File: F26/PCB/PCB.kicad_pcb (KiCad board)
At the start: 2 copper layers, 12 parts, among them J1 B3B-XH-A, J3 B2B-XH-A, J4 B3B-XH-A, J5 Conn_01x04, J6 Conn_01x06, J7 Conn_01x02, SW1 SW_Nidec_CAS-120A1, U4 815, U6 SC0194_9_

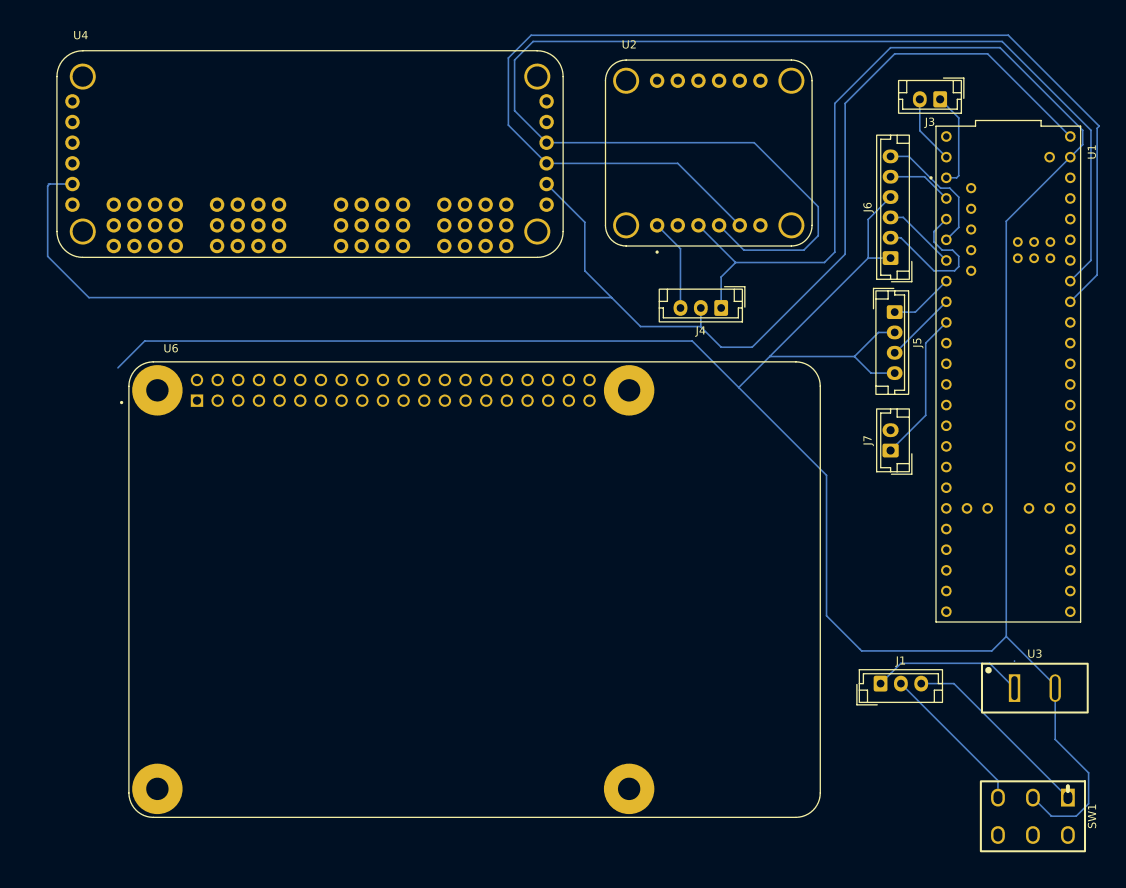
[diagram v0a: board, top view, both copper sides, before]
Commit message: PCB updates and Made wiring diagram
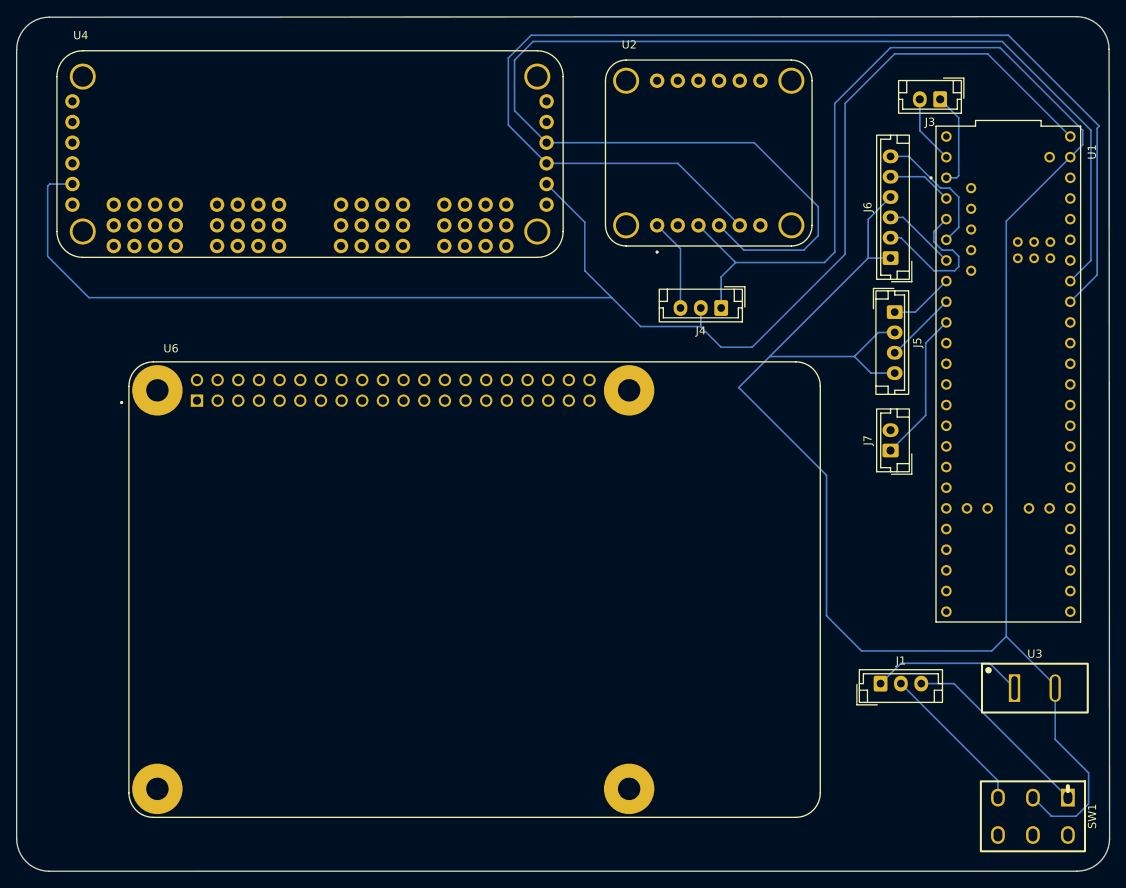
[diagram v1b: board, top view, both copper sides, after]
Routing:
- net Net-(J5-Pin_2): track 374.2 -> 294.1 mm
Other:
- board outline added: 134.4 x 105.1 mm
